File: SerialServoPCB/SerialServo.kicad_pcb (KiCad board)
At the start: 2 copper layers, 40.6 x 74.9 mm, 45 parts, among them J1 Conn_01x04, J2 Conn_01x05, J3 Conn_01x05, J4 Conn_01x03, SW1 SW_Push, SW2 SW_Push, SW3 SW_Push, U1 PIC16F1847-ISO, U2 LM358A, U3 L78L05_TO92, U4 LM7805_TO220

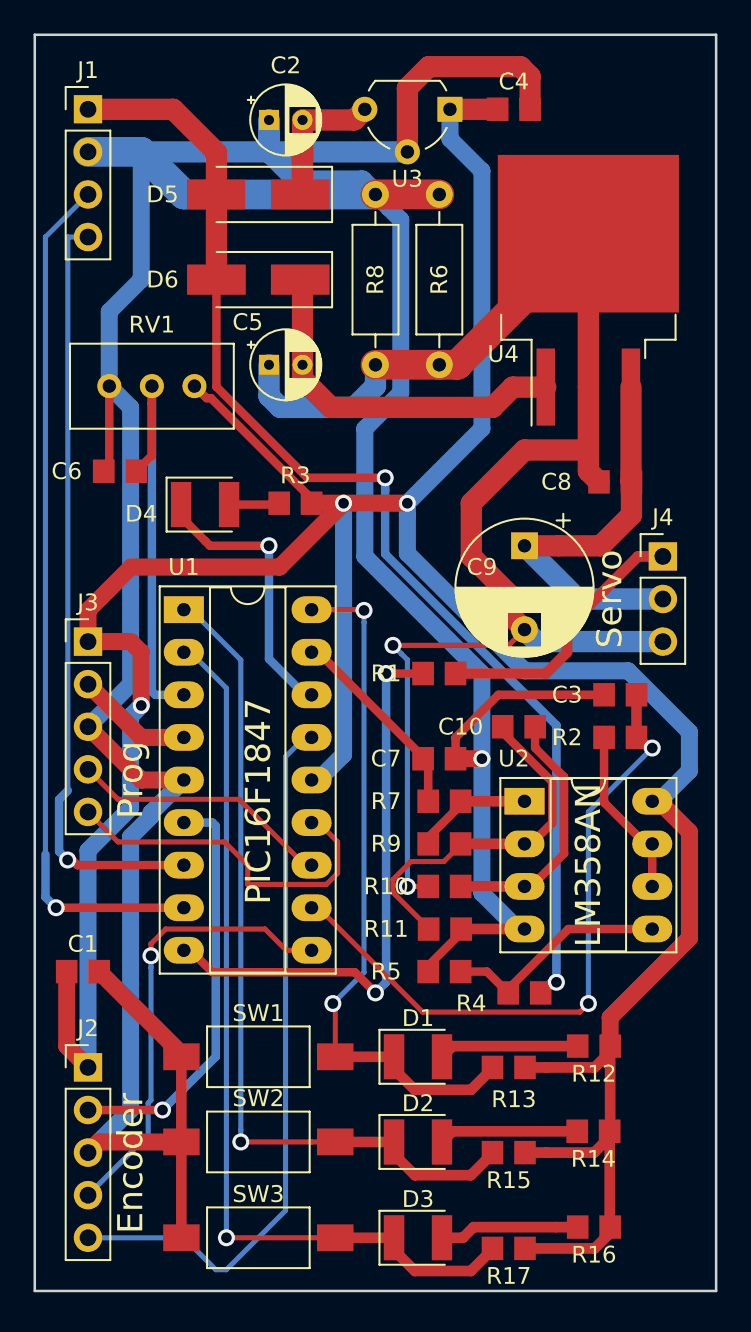
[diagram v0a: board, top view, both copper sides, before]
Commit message: PCb Rev A
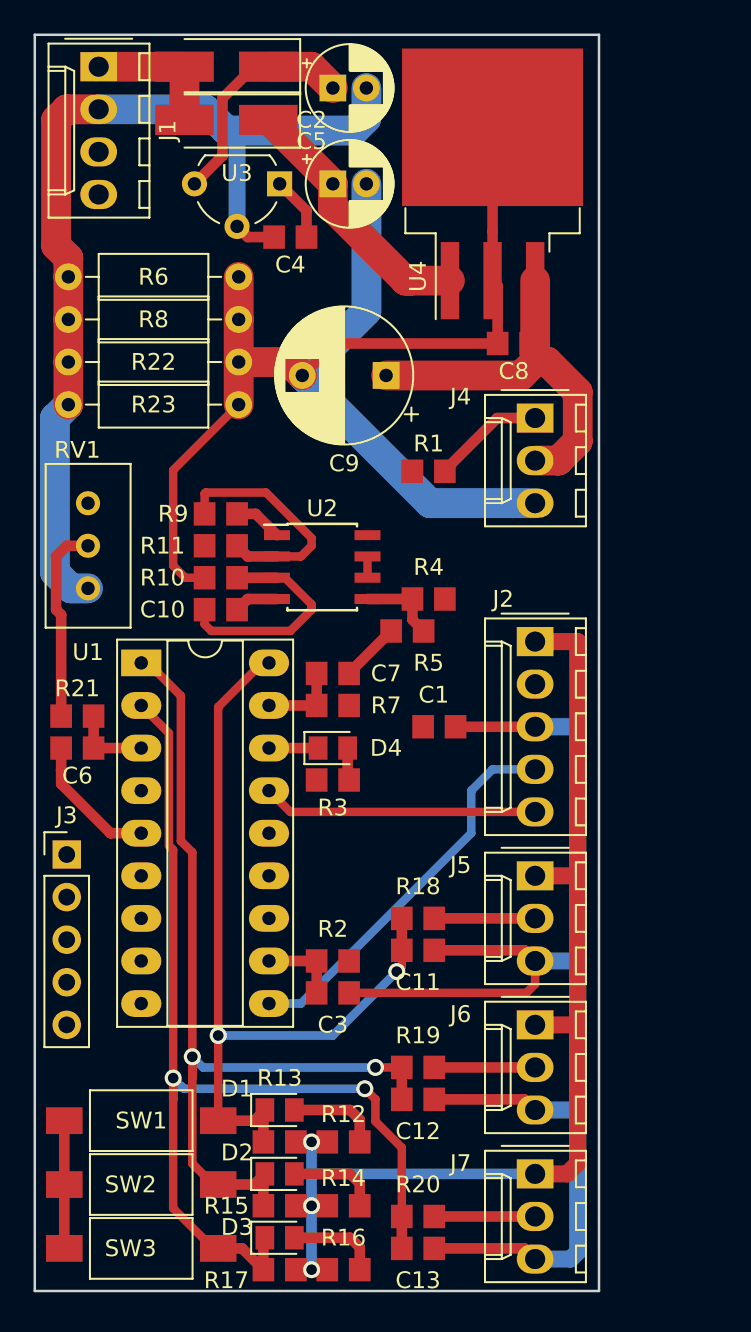
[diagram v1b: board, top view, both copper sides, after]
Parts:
- added C11: 0.1uF, Capacitor_SMD:C_0805_2012Metric_Pad1.29x1.40mm_HandSolder, F.Cu at (109.2, 120.7)
- added C12: 0.1uF, Capacitor_SMD:C_0805_2012Metric_Pad1.29x1.40mm_HandSolder, F.Cu at (109.2, 129.5)
- added C13: 0.1uF, Capacitor_SMD:C_0805_2012Metric_Pad1.29x1.40mm_HandSolder, F.Cu at (109.2, 138.4)
- added J5: Conn_01x03, Connector_Molex:Molex_KK-254_AE-6410-03A_1x03_P2.54mm_Vertical, F.Cu at (116.2, 116.2)
- added J6: Conn_01x03, Connector_Molex:Molex_KK-254_AE-6410-03A_1x03_P2.54mm_Vertical, F.Cu at (116.2, 125.1)
- added J7: Conn_01x03, Connector_Molex:Molex_KK-254_AE-6410-03A_1x03_P2.54mm_Vertical, F.Cu at (116.2, 134.0)
- added R18: 1K0, Resistor_SMD:R_0805_2012Metric_Pad1.29x1.40mm_HandSolder, F.Cu at (109.2, 118.7)
- added R19: 1K0, Resistor_SMD:R_0805_2012Metric_Pad1.29x1.40mm_HandSolder, F.Cu at (109.2, 127.6)
- added R20: 1K0, Resistor_SMD:R_0805_2012Metric_Pad1.29x1.40mm_HandSolder, F.Cu at (109.2, 136.5)
- added R21: 1K0, Resistor_SMD:R_0805_2012Metric_Pad1.29x1.40mm_HandSolder, F.Cu at (88.9, 106.7)
- added R22: 1R0, Resistor_THT:R_Axial_DIN0207_L6.3mm_D2.5mm_P10.16mm_Horizontal, F.Cu at (88.4, 85.6)
- added R23: 1R0, Resistor_THT:R_Axial_DIN0207_L6.3mm_D2.5mm_P10.16mm_Horizontal, F.Cu at (88.4, 88.1)
- C10: value 0.1uF -> 1uF
- C2, C5: footprint Capacitor_THT:CP_Radial_D4.0mm_P2.00mm -> Capacitor_THT:CP_Radial_D5.0mm_P2.00mm
- D1, D2, D3, D4: footprint LED_SMD:LED_1210_3225Metric_Pad1.22x2.70mm_HandSolder -> LED_SMD:LED_0805_2012Metric_Pad1.12x1.40mm_HandSolder
- J1: footprint Connector_PinHeader_2.54mm:PinHeader_1x04_P2.54mm_Vertical -> Connector_Molex:Molex_KK-254_AE-6410-04A_1x04_P2.54mm_Vertical
- J2: footprint Connector_PinHeader_2.54mm:PinHeader_1x05_P2.54mm_Vertical -> Connector_Molex:Molex_KK-254_AE-6410-05A_1x05_P2.54mm_Vertical
- J4: footprint Connector_PinHeader_2.54mm:PinHeader_1x03_P2.54mm_Vertical -> Connector_Molex:Molex_KK-254_AE-6410-03A_1x03_P2.54mm_Vertical
- R10: value 10K -> 47K
- U2: footprint Package_DIP:DIP-8_W7.62mm_Socket_LongPads -> Package_SO:SOIC-8_3.9x4.9mm_P1.27mm
- moved J2 36.8 mm to (116.2, 102.2), turned to 270 degrees
- moved R11 26.5 mm to (97.5, 96.5), turned to 0 degrees
- moved C1 25.8 mm to (110.5, 107.3)
- moved C3 24.7 mm to (104.1, 123.2), turned to 0 degrees
- moved R4 24.2 mm to (109.9, 99.7)
- moved R9 23.8 mm to (97.5, 94.6), turned to 0 degrees
- moved R10 22.7 mm to (97.5, 98.4)
- moved R6 22.7 mm to (88.4, 80.5), turned to 0 degrees
- moved R2 21.7 mm to (104.1, 121.3), turned to 180 degrees
- moved R5 20.4 mm to (108.6, 101.6)
- moved R8 19.8 mm to (88.4, 83.0), turned to 0 degrees
- moved C10 19.1 mm to (97.5, 100.3), turned to 0 degrees
- moved U2 18.5 mm to (103.5, 97.8)
- moved C6 16.7 mm to (88.9, 108.6)
- moved R3 16.7 mm to (104.1, 110.5), turned to 180 degrees
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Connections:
- C10 pad 2: Net-(C10-Pad2) -> GND
- C2 pad 1: GND -> Net-(C2-Pad1)
- C2 pad 2: Net-(C2-Pad2) -> GND
- C5 pad 1: GNDA -> Net-(C5-Pad1)
- C5 pad 2: Net-(C5-Pad2) -> GNDA
- D5 pad 1: Net-(C2-Pad2) -> Net-(C2-Pad1)
- D6 pad 1: Net-(C5-Pad2) -> Net-(C5-Pad1)
- R11 pad 2: Net-(C10-Pad2) -> Net-(R11-Pad2)
- R9 pad 1: Net-(C10-Pad2) -> Net-(R11-Pad2)
- RV1 pad 2: /AN4 -> Net-(R21-Pad1)
- U2 pad 2: Net-(C10-Pad2) -> Net-(R11-Pad2)
- U3 pad 3: Net-(C2-Pad2) -> Net-(C2-Pad1)
- U4 pad 1: Net-(C5-Pad2) -> Net-(C5-Pad1)
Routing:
- net +5V: track 193.2 -> 72.0 mm
- net GND: track 229.6 -> 159.8 mm, vias 1 -> 0
- net +12V: track 70.5 -> 8.30 mm, vias 2 -> 0
- net TX: track 51.5 -> 0.00 mm, vias 1 -> 0
- net RX: track 45.8 -> 0.00 mm, vias 1 -> 0
- net Batt_V: track 39.9 -> 4.75 mm, vias 2 -> 0
- net Net-(R1-Pad1): track 34.0 -> 0.00 mm, vias 2 -> 0
- net Enc_DO: track 43.1 -> 16.4 mm
- net ENC_CS: track 24.7 -> 0.00 mm, vias 1 -> 0
- net Net-(C10-Pad2): track 21.7 -> 0.00 mm
- net Net-(C5-Pad2): track 21.7 -> 0.00 mm
- net PGD: track 21.5 -> 0.00 mm
- net /AN4: track 25.7 -> 4.75 mm
- net PGC: track 15.7 -> 0.00 mm
- net Net-(C5-Pad1): track 0.00 -> 15.6 mm
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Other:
- board size 40.6 x 74.9 mm -> 33.7 x 74.9 mm
- board text removed: "DMFE 2018"
- board text removed: "Encoder"
- board text removed: "LM358AN"
- board text removed: "PIC16F1847"
- board text removed: "Prog"
- board text removed: "Serial Servo Rev n/c"
- board text removed: "Servo"
